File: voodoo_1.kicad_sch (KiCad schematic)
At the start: 1 part, among them U1 LM301

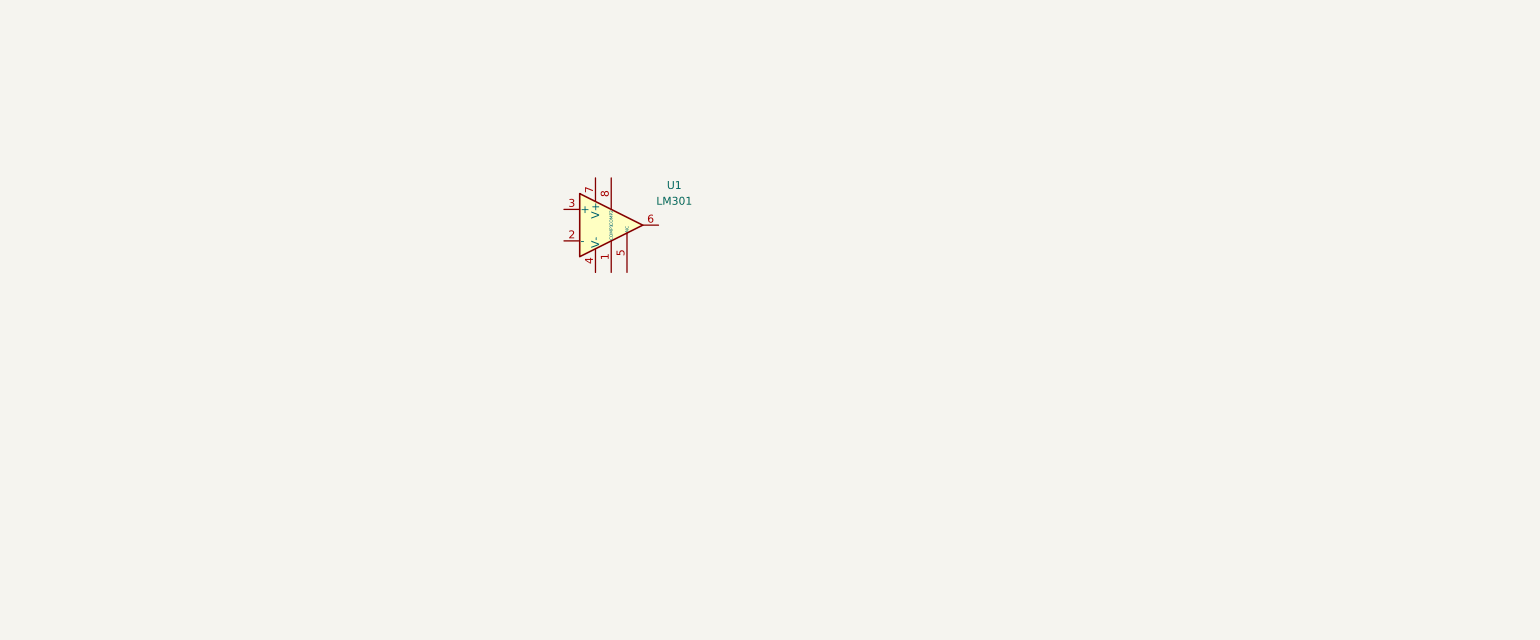
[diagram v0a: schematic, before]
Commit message: 回路図作成
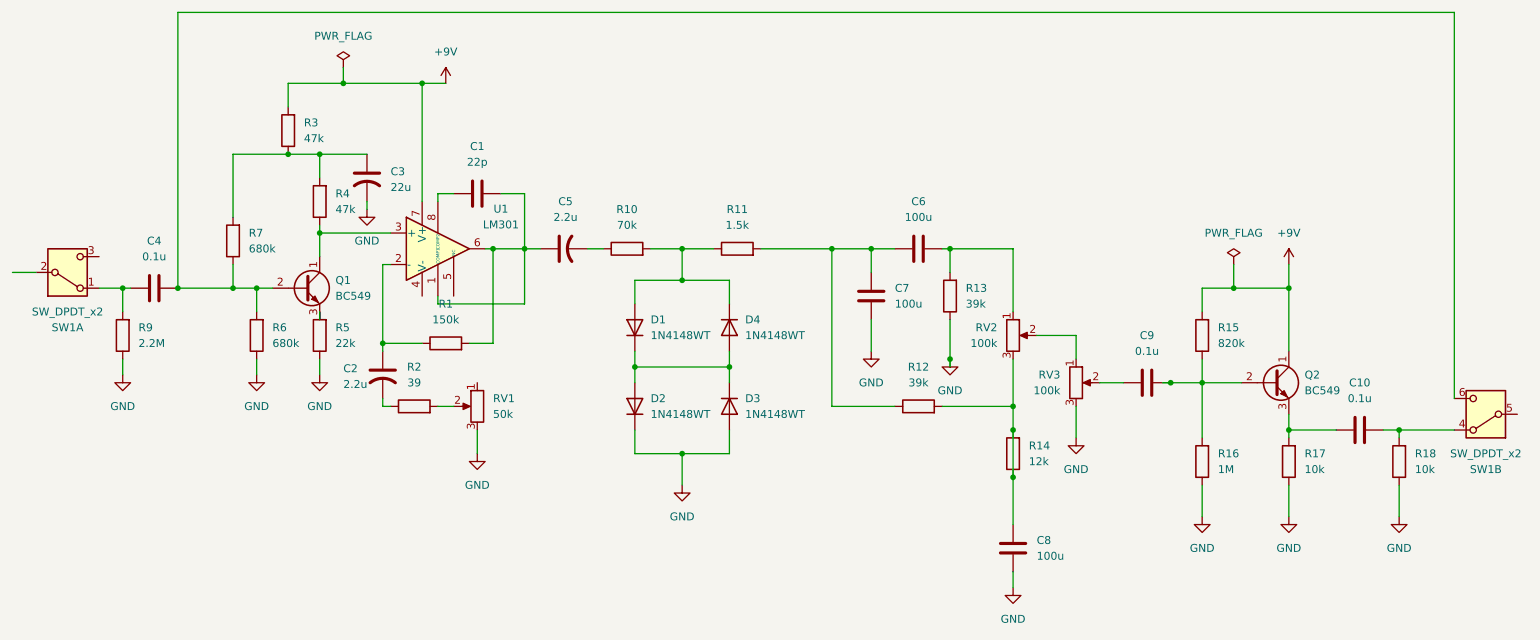
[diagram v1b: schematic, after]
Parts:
- added C1: 22p, symbol Device:C
- added C10, C4, C9: 0.1u, symbol Device:C
- added C2, C5: 2.2u, symbol Device:C_US
- added C3: 22u, symbol Device:C_US
- added C6, C7, C8: 100u, symbol Device:C
- added D1, D2, D3, D4: 1N4148WT, Diode_SMD:D_SOD-523, symbol Diode:1N4148WT
- added Q1, Q2: BC549, Package_TO_SOT_THT:TO-92_Inline, symbol Transistor_BJT:BC549
- added R1: 150k, symbol Device:R
- added R10: 70k, symbol Device:R
- added R11: 1.5k, symbol Device:R
- added R12, R13: 39k, symbol Device:R
- added R14: 12k, symbol Device:R
- added R15: 820k, symbol Device:R
- added R16: 1M, symbol Device:R
- added R17, R18: 10k, symbol Device:R
- added R2: 39, symbol Device:R
- added R3, R4: 47k, symbol Device:R
- added R5: 22k, symbol Device:R
- added R6, R7: 680k, symbol Device:R
- added R9: 2.2M, symbol Device:R
- added RV1: 50k, symbol Device:R_Potentiometer
- added RV2, RV3: 100k, symbol Device:R_Potentiometer
- added SW1: SW_DPDT_x2, symbol Switch:SW_DPDT_x2
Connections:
- net at U1.1 (COMP1): now also U1.6, C1.1, C5.1, R1.2
- net at U1.2 (-): now also C2.1, R1.1
- net at U1.3 (+): now also Q1.1 (C), R4.1
- net +9V: now reaches U1.7 (V+)
- net +9V: now also Q2.1 (C), R15.2, R3.2
- net at U1.8 (COMP2): now also C1.2
- new net: D1.1 (K), D2.2 (A), D3.1 (K), D4.2 (A)
- new net: D1.2 (A), D4.1 (K), R10.2, R11.1
- new net: C6.2, C7.1, R11.2, R12.1
- new net: C8.1, R12.2, R14.1, R14.2, RV2.3
- new net: C6.1, R13.2, RV2.1
- new net: C9.1, Q2.2 (B), R15.1, R16.2
- new net: RV2.2, RV3.1
- new net: C9.2, RV3.2
- new net: C4.1, Q1.2 (B), R6.2, R7.1, SW1.6 (C)
- new net: C3.1, R3.1, R4.2, R7.2
- new net: C10.1, R18.2, SW1.4 (A)
- new net: C10.2, Q2.3 (E), R17.2
- new net: C5.2, R10.1
- new net: C2.2, R2.1
- new net: R2.2, RV1.2
- new net: C4.2, R9.2, SW1.1 (A)
- new net: Q1.3 (E), R5.2
- new net GND: C3.2, C7.2, C8.2, D2.1 (K), D3.2 (A), R13.1, R16.1, R17.1, R18.1, R5.1, R6.1, R9.1, RV1.3, RV3.3
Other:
- moved on the sheet: U1
